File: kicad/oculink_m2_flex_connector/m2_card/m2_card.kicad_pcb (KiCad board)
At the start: 2 copper layers, 22 x 4.2 mm, 18 parts, among them J1 G14A42121B12HR

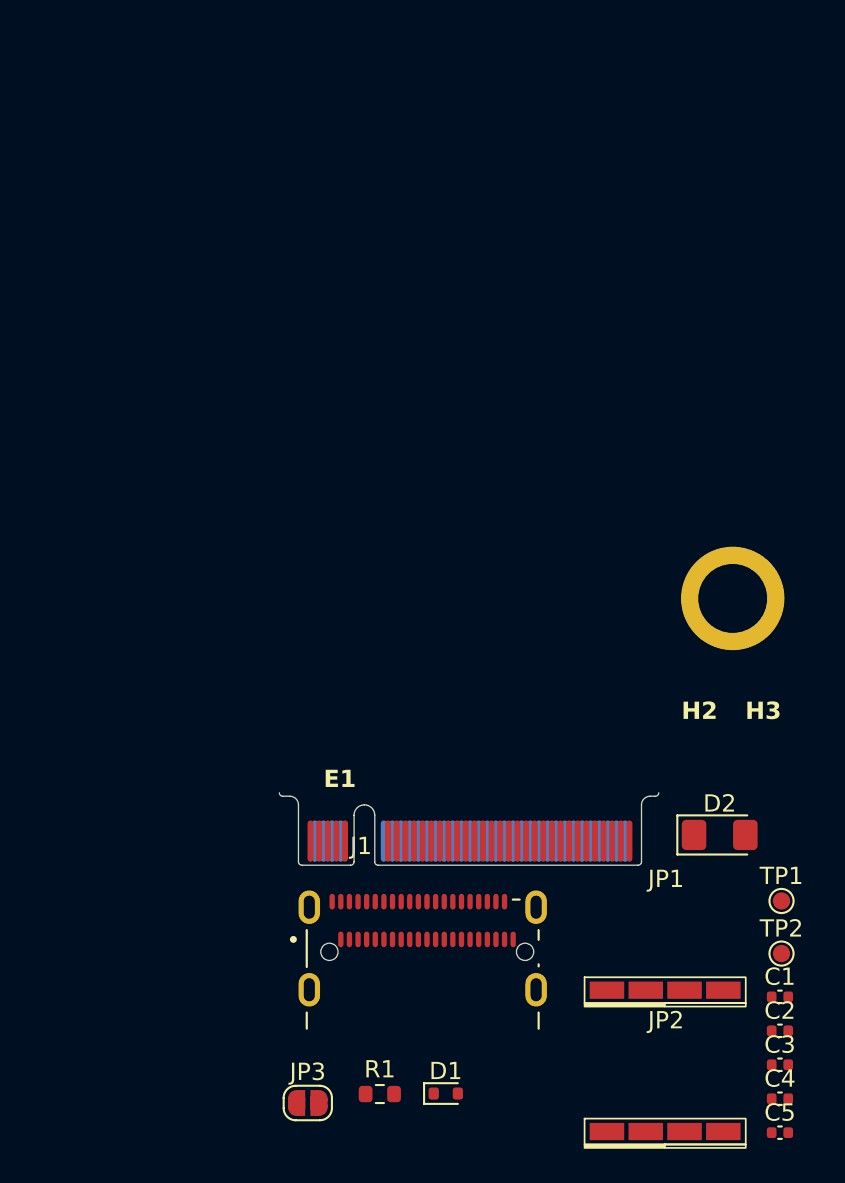
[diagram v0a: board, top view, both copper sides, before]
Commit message: Finished first draft of m2 card
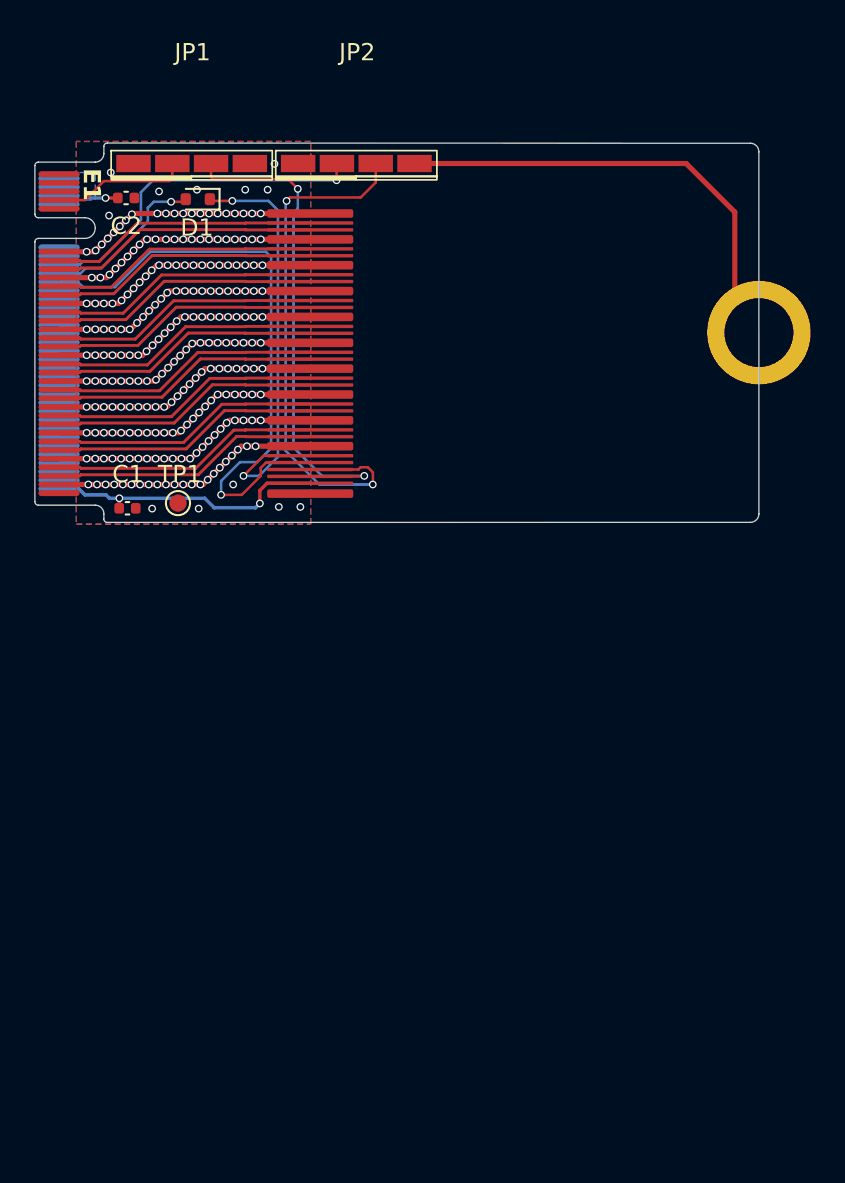
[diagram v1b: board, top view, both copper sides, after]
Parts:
- removed C3, C4, C5: 100n, Capacitor_SMD:C_0402_1005Metric
- removed D2: Power LED, LED_SMD:LED_1206_3216Metric_Pad1.42x1.75mm_HandSolder
- removed H2: MOUNT_1, custom_edge_connector:secondary_mounting_hole
- removed H3: MOUNT_2, custom_edge_connector:secondary_mounting_hole
- removed JP3: JMP_3.3V_EXT, Jumper:SolderJumper-2_P1.3mm_Open_RoundedPad1.0x1.5mm
- removed R1: 100, Resistor_SMD:R_0603_1608Metric
- removed TP2: TP_GND_2, TestPoint:TestPoint_Pad_D1.0mm
- J1: value G14A42121B12HR -> Conn_01x38_Pin; footprint amphenol_oculink:AMPHENOL_G14A42121B12HR -> flex_connector:port_pcb; moved to B.Cu
- moved C2 61.4 mm to (107.8, 67.7), turned to 180 degrees
- moved JP2 58.9 mm to (121.2, 59.7)
- moved JP1 55.3 mm to (111.6, 59.7)
- moved D1 53.8 mm to (112.0, 67.8), turned to 180 degrees
- moved J1 48.1 mm to (118.5, 63.7), turned to 180 degrees
- moved C1 47.3 mm to (107.9, 85.7)
- moved TP1 41.9 mm to (110.8, 85.4)
- moved H1 15.5 mm to (144.5, 75.5)
- moved E1 14.1 mm to (121.0, 75.5), turned to -90 degrees
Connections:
- C2 pad 1: +3.3V -> GND
- C2 pad 2: GND -> +3.3V0
- E1 pad 12: +3.3V -> unconnected-(E1-3.3V-Pad12)
- E1 pad 14: +3.3V -> unconnected-(E1-3.3V-Pad14)
- E1 pad 16: +3.3V -> unconnected-(E1-3.3V-Pad16)
- E1 pad 18: +3.3V -> unconnected-(E1-3.3V-Pad18)
- E1 pad 4: +3.3V -> unconnected-(E1-3.3V-Pad4)
- E1 pad 70: +3.3V -> +3.3V0
- E1 pad 72: +3.3V -> +3.3V0
- E1 pad 74: +3.3V -> +3.3V0
- JP1 pad 3: /PEDET_EXT -> Net-(J1-Pin_32)
- JP2 pad 3: /PEWAKE_EXT -> Net-(J1-Pin_31)
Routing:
- net GND: track 0.00 -> 181.3 mm, vias 0 -> 238
- net PERST: track 0.00 -> 35.2 mm, vias 0 -> 1
- net Net-(J1-Pin_31): track 0.00 -> 31.6 mm, vias 0 -> 2
- net Net-(J1-Pin_32): track 0.00 -> 29.1 mm, vias 0 -> 2
- net /CLKREQ_EXT: track 0.00 -> 25.3 mm, vias 0 -> 2
- net PEWAKE: track 0.00 -> 20.0 mm, vias 0 -> 1
- net +3.3V: track 0.00 -> 16.6 mm, vias 0 -> 2
- net TX3+: track 0.00 -> 15.5 mm
- net TX2+: track 0.00 -> 15.5 mm
- net TX1+: track 0.00 -> 15.5 mm
- net TX0+: track 0.00 -> 15.5 mm
- net RX3+: track 0.00 -> 15.5 mm
- net RX2+: track 0.00 -> 15.5 mm
- net RX1+: track 0.00 -> 15.5 mm
- net RX0+: track 0.00 -> 15.5 mm
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- added copper zone on B.Cu, net +3.3V0
- added copper zone on B.Cu, net GND
- added copper zone on F.Cu, net GND
- added copper zone on In1.Cu, net GND
- added copper zone on In2.Cu, net GND
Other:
- board size 22 x 4.2 mm -> 37.8 x 22 mm
- copper layers 2 -> 4
